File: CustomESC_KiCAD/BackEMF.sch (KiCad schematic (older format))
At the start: 13 parts, among them U4 LM339

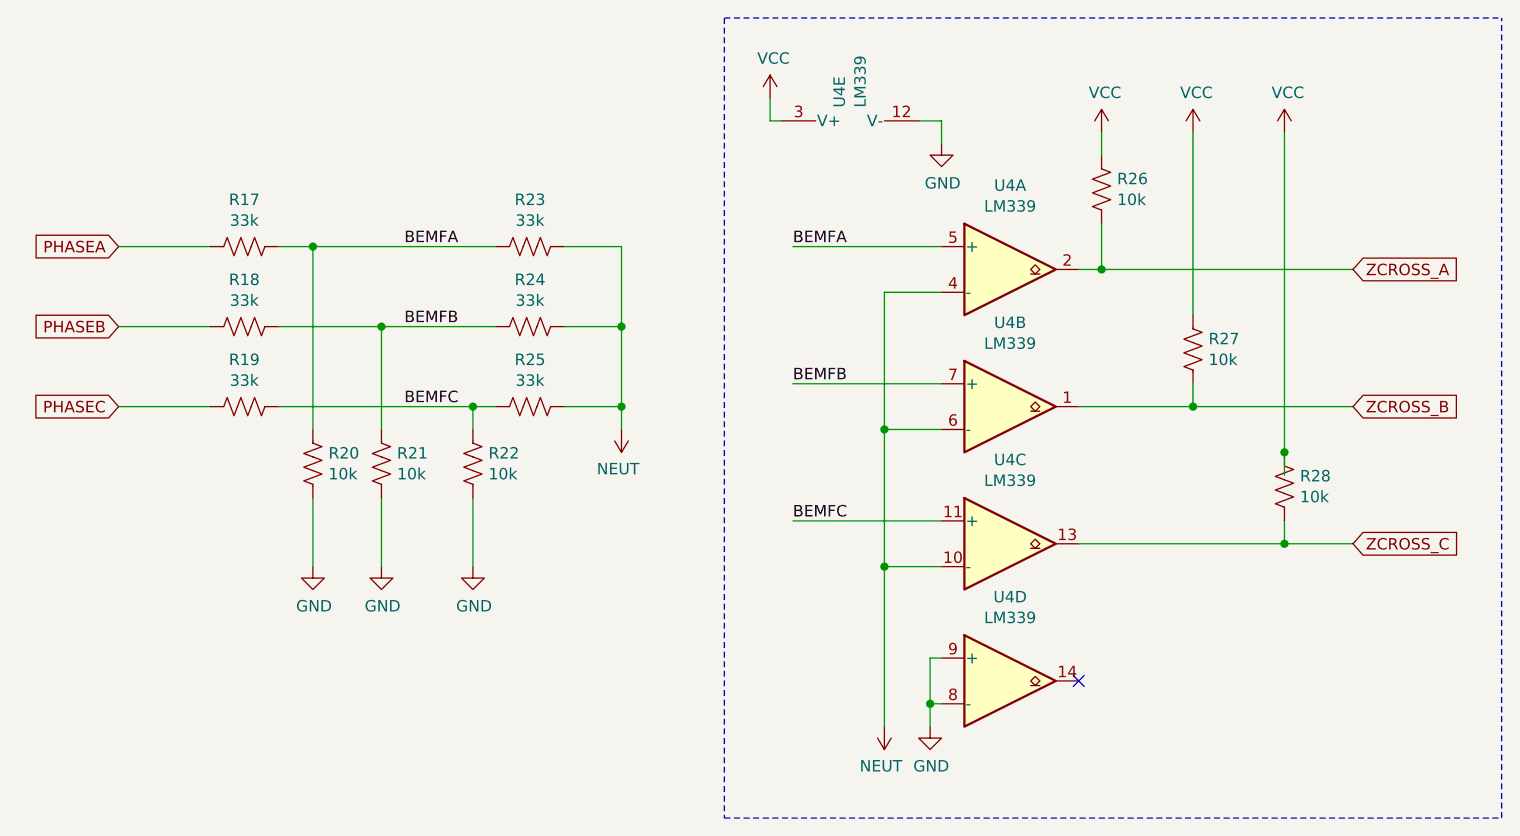
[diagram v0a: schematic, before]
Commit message: Finish Custom ESC layout
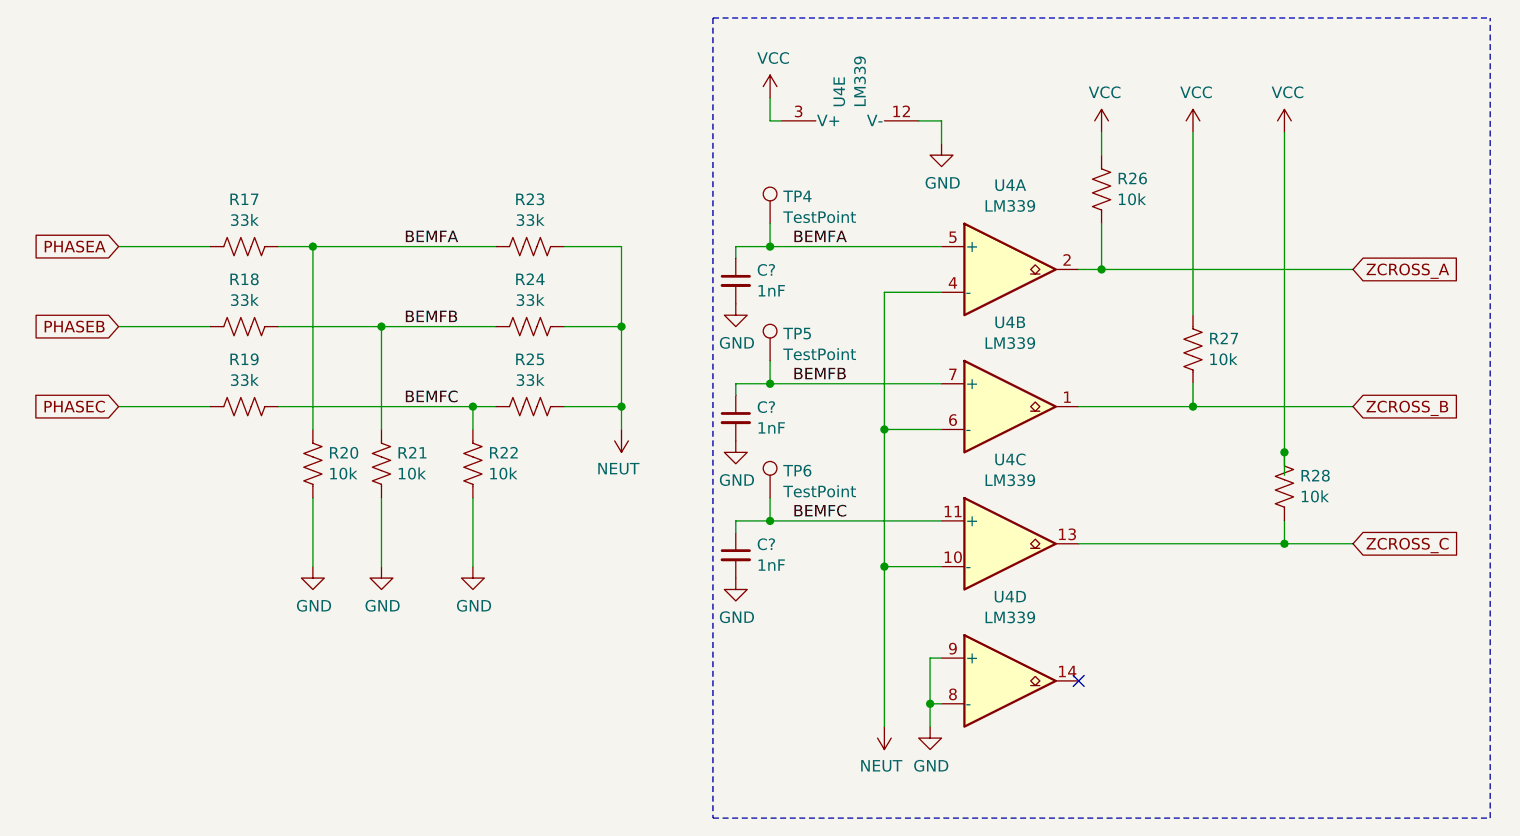
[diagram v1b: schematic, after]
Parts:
- added C? (x3): 1nF, symbol Device:C_Small
- added TP4, TP5, TP6: TestPoint, TestPoint:TestPoint_Pad_D1.0mm, symbol Connector:TestPoint
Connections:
- net BEMFA: now also C?.1, TP4.1
- net BEMFB: now also C?.1, TP5.1
- net BEMFC: now also C?.1, TP6.1
- net GND: now also C?.2, C?.2, C?.2
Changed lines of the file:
@@
 Text Label 6100 2750 0    50   ~ 0
 BEMFA
-Wire Wire Line
-	6100 2750 6750 2750
 Text Label 6100 3350 0    50   ~ 0
 BEMFB
-Wire Wire Line
-	6100 3350 6750 3350
 Text Label 6100 3950 0    50   ~ 0
 BEMFC
-Wire Wire Line
-	6100 3950 6750 3950
 $Comp
 L power:VCC #PWR031
@@
 NoConn ~ 7350 4650
 Wire Notes Line
-	5800 1750 5800 5250
+	5750 1750 5750 5250
 Text GLabel 8550 4050 2    50   Input ~ 0
 ZCROSS_C
@@
 	8250 3950 8250 4050
 Wire Notes Line
-	9200 5250 9200 1750
-Wire Notes Line
-	5800 5250 9200 5250
-Wire Notes Line
-	5800 1750 9200 1750
+	9150 5250 9150 1750
+Wire Notes Line
+	5750 5250 9150 5250
+Wire Notes Line
+	5750 1750 9150 1750
+$Comp
+L Connector:TestPoint TP4
+U 1 1 617766C1
+P 6000 2650
+F 0 "TP4" H 6058 2768 50  0000 L CNN
+F 1 "TestPoint" H 6058 2677 50  0000 L CNN
+F 2 "TestPoint:TestPoint_Pad_D1.0mm" H 6200 2650 50  0001 C CNN
+F 3 "~" H 6200 2650 50  0001 C CNN
+	1    6000 2650
+	1    0    0    -1
+$EndComp
+Wire Wire Line
+	6000 2650 6000 2750
+Wire Wire Line
+	6000 2750 6750 2750
+$Comp
+L Connector:TestPoint TP5
+U 1 1 61777EA6
+P 6000 3250
+F 0 "TP5" H 6058 3368 50  0000 L CNN
+F 1 "TestPoint" H 6058 3277 50  0000 L CNN
+F 2 "TestPoint:TestPoint_Pad_D1.0mm" H 6200 3250 50  0001 C CNN
+F 3 "~" H 6200 3250 50  0001 C CNN
+	1    6000 3250
+	1    0    0    -1
+$EndComp
+Wire Wire Line
+	6000 3250 6000 3350
+Wire Wire Line
+	6000 3350 6750 3350
+$Comp
+L Connector:TestPoint TP6
+U 1 1 6177979B
+P 6000 3850
+F 0 "TP6" H 6058 3968 50  0000 L CNN
+F 1 "TestPoint" H 6058 3877 50  0000 L CNN
+F 2 "TestPoint:TestPoint_Pad_D1.0mm" H 6200 3850 50  0001 C CNN
+F 3 "~" H 6200 3850 50  0001 C CNN
+	1    6000 3850
+	1    0    0    -1
+$EndComp
+Wire Wire Line
+	6000 3850 6000 3950
+Wire Wire Line
+	6000 3950 6750 3950
+$Comp
+L Device:C_Small C?
+U 1 1 617F77EE
+P 5850 3500
+F 0 "C?" H 5942 3546 50  0000 L CNN
+F 1 "1nF" H 5942 3455 50  0000 L CNN
+F 2 "" H 5850 3500 50  0001 C CNN
+F 3 "~" H 5850 3500 50  0001 C CNN
+	1    5850 3500
+	1    0    0    -1
+$EndComp
+$Comp
+L Device:C_Small C?
+U 1 1 617F7DE6
+P 5850 4100
+F 0 "C?" H 5942 4146 50  0000 L CNN
+F 1 "1nF" H 5942 4055 50  0000 L CNN
+F 2 "" H 5850 4100 50  0001 C CNN
+F 3 "~" H 5850 4100 50  0001 C CNN
+	1    5850 4100
+	1    0    0    -1
+$EndComp
+Wire Wire Line
+	5850 4000 5850 3950
+Wire Wire Line
+	5850 3950 6000 3950
+Connection ~ 6000 3950
+Wire Wire Line
+	5850 3400 5850 3350
+Wire Wire Line
+	5850 3350 6000 3350
+Connection ~ 6000 3350
+$Comp
+L power:GND #PWR?
+U 1 1 61802A49
+P 5850 4200
+F 0 "#PWR?" H 5850 3950 50  0001 C CNN
+F 1 "GND" H 5855 4027 50  0000 C CNN
+F 2 "" H 5850 4200 50  0001 C CNN
+F 3 "" H 5850 4200 50  0001 C CNN
+	1    5850 4200
+	1    0    0    -1
+$EndComp
+$Comp
+L power:GND #PWR?
+U 1 1 6180313E
+P 5850 3600
+F 0 "#PWR?" H 5850 3350 50  0001 C CNN
+F 1 "GND" H 5855 3427 50  0000 C CNN
+F 2 "" H 5850 3600 50  0001 C CNN
+F 3 "" H 5850 3600 50  0001 C CNN
+	1    5850 3600
+	1    0    0    -1
+$EndComp
+$Comp
+L power:GND #PWR?
+U 1 1 61803753
+P 5850 3000
+F 0 "#PWR?" H 5850 2750 50  0001 C CNN
+F 1 "GND" H 5855 2827 50  0000 C CNN
+F 2 "" H 5850 3000 50  0001 C CNN
+F 3 "" H 5850 3000 50  0001 C CNN
+	1    5850 3000
+	1    0    0    -1
+$EndComp
+$Comp
+L Device:C_Small C?
+U 1 1 618072A2
+P 5850 2900
+F 0 "C?" H 5942 2946 50  0000 L CNN
+F 1 "1nF" H 5942 2855 50  0000 L CNN
+F 2 "" H 5850 2900 50  0001 C CNN
+F 3 "~" H 5850 2900 50  0001 C CNN
+	1    5850 2900
+	1    0    0    -1
+$EndComp
+Wire Wire Line
+	6000 2750 5850 2750
+Wire Wire Line
+	5850 2750 5850 2800
+Connection ~ 6000 2750
 $EndSCHEMATC
